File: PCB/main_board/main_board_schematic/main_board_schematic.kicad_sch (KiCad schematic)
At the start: 6 parts, among them P1 USB_C_Plug_USB2.0, U1 NCP1117-3.3_SOT223

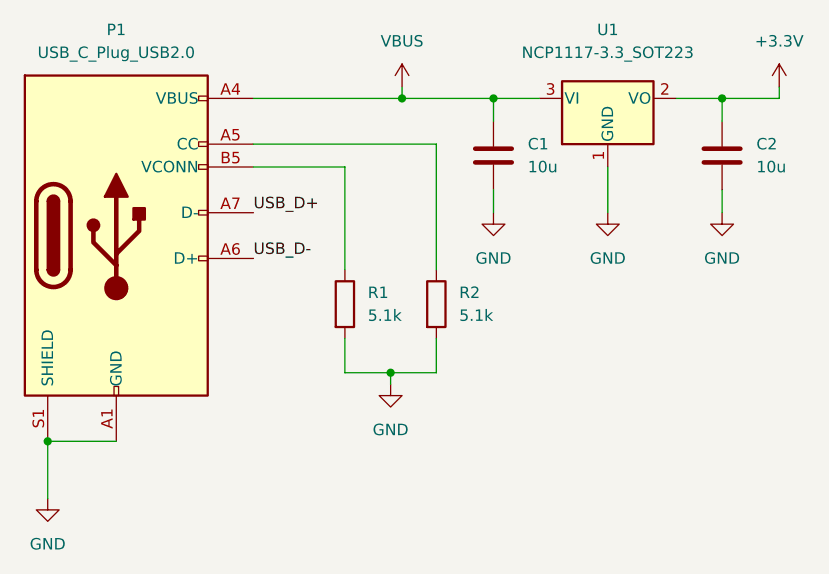
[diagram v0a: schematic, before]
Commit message: Fixed wiring mistake...
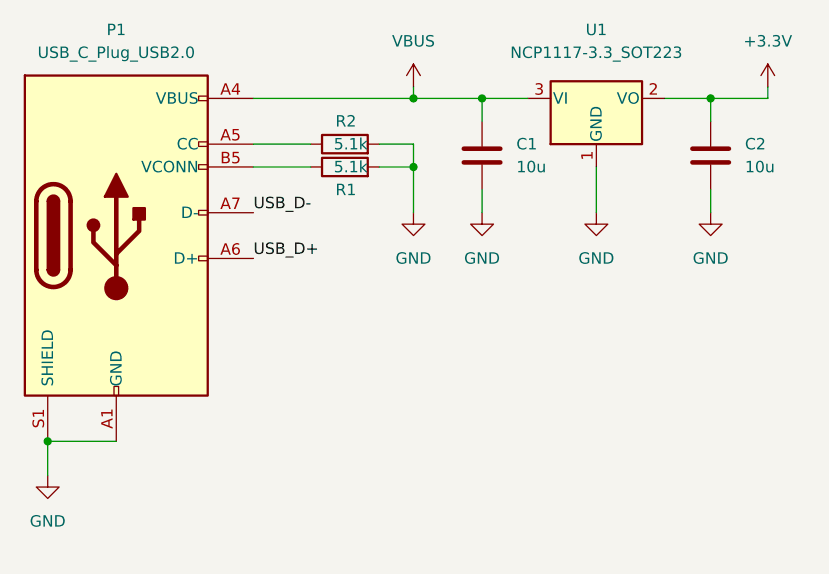
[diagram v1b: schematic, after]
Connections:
- net USB_D+: now also P1.A6 (D+); no longer P1.A7 (D-)
- net USB_D-: now also P1.A7 (D-); no longer P1.A6 (D+)
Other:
- moved on the sheet: C1, C2, R1, R2, U1
